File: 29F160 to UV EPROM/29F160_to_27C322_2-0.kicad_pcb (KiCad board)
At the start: 4 copper layers, 54.4 x 17.8 mm, 14 parts, among them U1 27C322, U2 29F160, U3 29F160, U4 74LS139

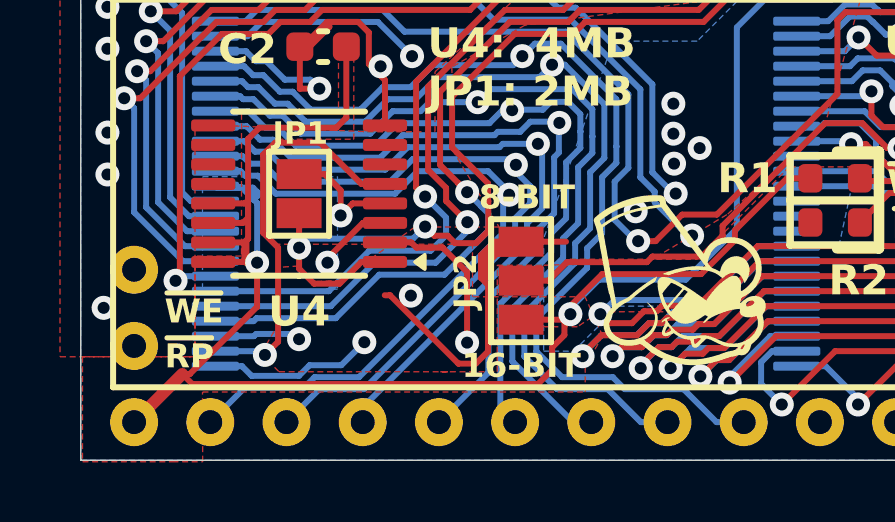
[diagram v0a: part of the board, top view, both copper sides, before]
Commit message: Add files via upload
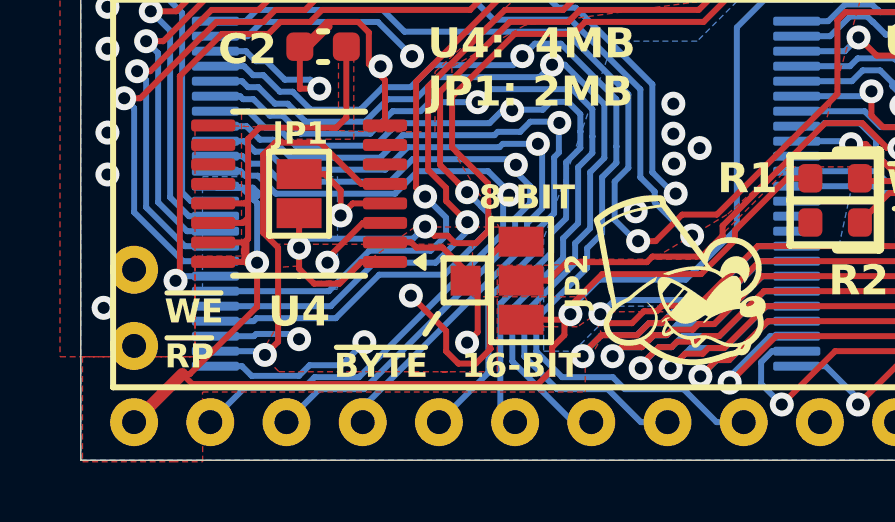
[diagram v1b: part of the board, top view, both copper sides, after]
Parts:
- added TP3: TPB1,27, TestPoint:TestPoint_Pad_1.0x1.0mm, F.Cu at (183.8, 102.0)
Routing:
- net GND: track 74.0 -> 64.2 mm
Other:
- board text added: "~{BYTE}"
